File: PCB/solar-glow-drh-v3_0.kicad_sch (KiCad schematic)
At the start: 57 parts, among them J1 UPDI hdr, Q1 BCP5316MTWG, SW2 LED master, U1 AVR64DD28 (VQFN28), U2 ALD910025SALI, U3 LIS2DH12, U4 TLV3011BIDBVR, U5 NT3H2211, U6 TPS22918

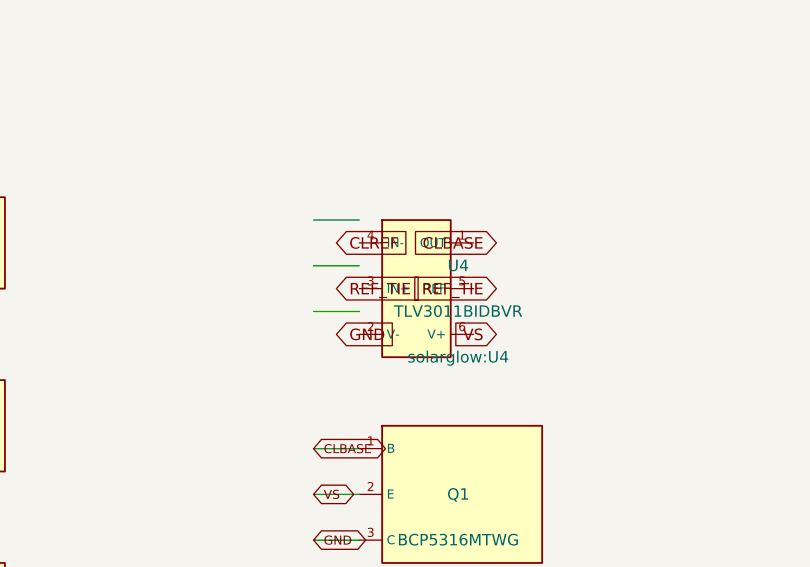
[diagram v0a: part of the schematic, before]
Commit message: Add files via upload
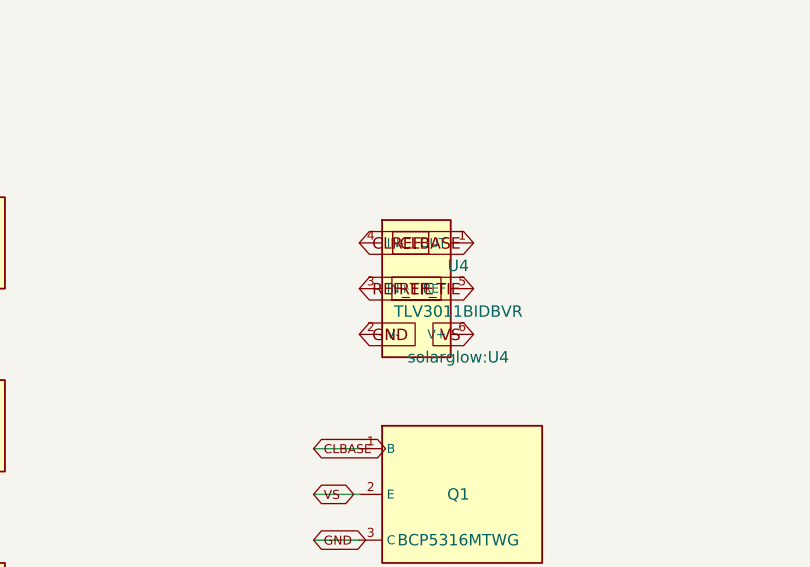
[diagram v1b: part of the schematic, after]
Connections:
- net CLBASE: now also U4.1 (OUT)
- net CLREF: now also U4.4 (IN-)
- net GND: now also U4.2 (V-)
- net REF_TIE: now also U4.3 (IN+), U4.5 (REF)
- net VS: now also U4.6 (V+)
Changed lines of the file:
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@@
 	(wire
 		(pts
-			(xy 139.7 38.1) (xy 134.62 38.1)
-		)
-		(stroke
-			(width 0)
-			(type default)
-		)
-	)
-	(wire
-		(pts
 			(xy 350.52 58.42) (xy 345.44 58.42)
 		)
@@
 	(wire
 		(pts
-			(xy 139.7 48.26) (xy 134.62 48.26)
-		)
-		(stroke
-			(width 0)
-			(type default)
-		)
-	)
-	(wire
-		(pts
 			(xy 209.55 58.42) (xy 204.47 58.42)
 		)
@@
 	(wire
 		(pts
-			(xy 139.7 43.18) (xy 134.62 43.18)
-		)
-		(stroke
-			(width 0)
-			(type default)
-		)
-	)
-	(wire
-		(pts
 			(xy 350.52 93.98) (xy 345.44 93.98)
 		)
@@
 	(global_label "CLREF"
 		(shape input)
-		(at 137.16 40.64 0)
+		(at 139.7 40.64 0)
 		(effects
 			(font
@@
 		)
 		(property "Intersheetrefs" "${INTERSHEET_REFS}"
-			(at 137.16 40.64 0)
+			(at 139.7 40.64 0)
 			(hide yes)
 			(show_name no)
@@
 	(global_label "REF_TIE"
 		(shape input)
-		(at 154.94 45.72 180)
+		(at 152.4 45.72 180)
 		(effects
 			(font
@@
 	(global_label "VS"
 		(shape input)
-		(at 154.94 50.8 180)
+		(at 152.4 50.8 180)
 		(effects
 			(font
@@
 	(global_label "CLBASE"
 		(shape input)
-		(at 154.94 40.64 180)
+		(at 152.4 40.64 180)
 		(effects
 			(font
@@
 	(global_label "GND"
 		(shape input)
-		(at 137.16 50.8 0)
+		(at 139.7 50.8 0)
 		(effects
 			(font
@@
 		)
 		(property "Intersheetrefs" "${INTERSHEET_REFS}"
-			(at 137.16 50.8 0)
+			(at 139.7 50.8 0)
 			(hide yes)
 			(show_name no)
@@
 	(global_label "REF_TIE"
 		(shape input)
-		(at 137.16 45.72 0)
+		(at 139.7 45.72 0)
 		(effects
 			(font
@@
 		)
 		(property "Intersheetrefs" "${INTERSHEET_REFS}"
-			(at 137.16 45.72 0)
+			(at 139.7 45.72 0)
 			(hide yes)
 			(show_name no)
